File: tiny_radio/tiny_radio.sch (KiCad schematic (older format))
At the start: 9 parts, among them IC1 ATTINY84-P, P1 CONN_4, P2 CONN_3X2, P3 CONN_2, U1 RFM12B

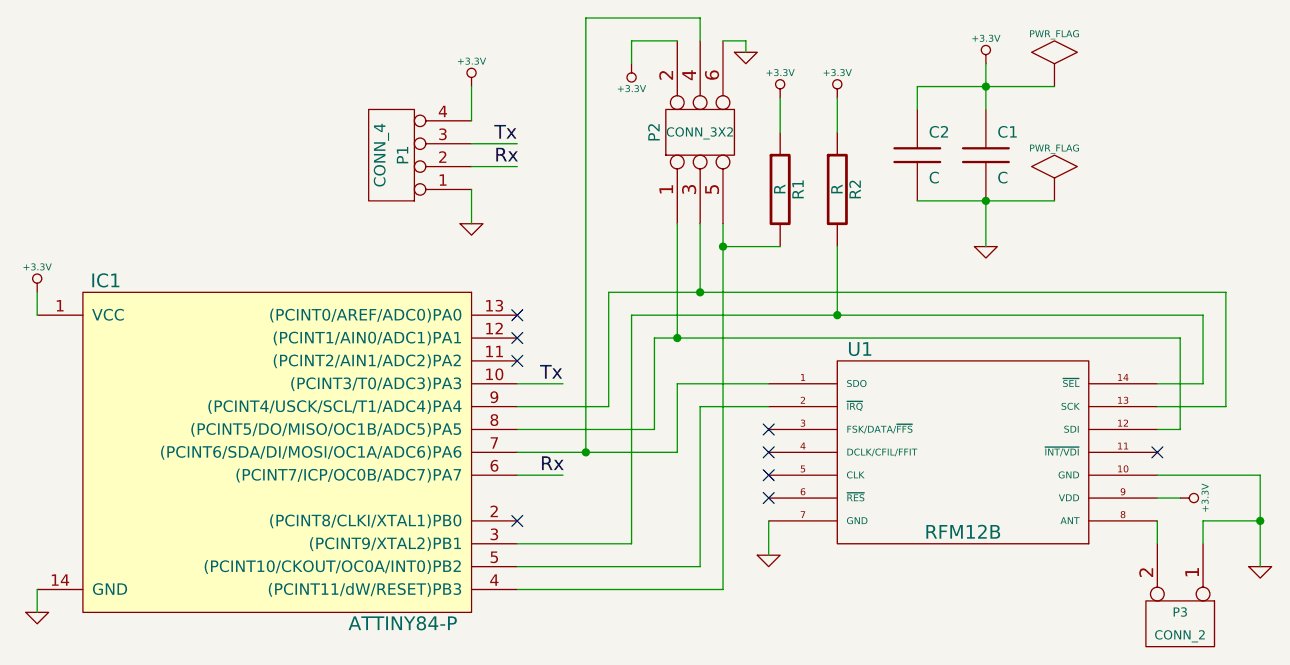
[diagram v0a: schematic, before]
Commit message: moved block over
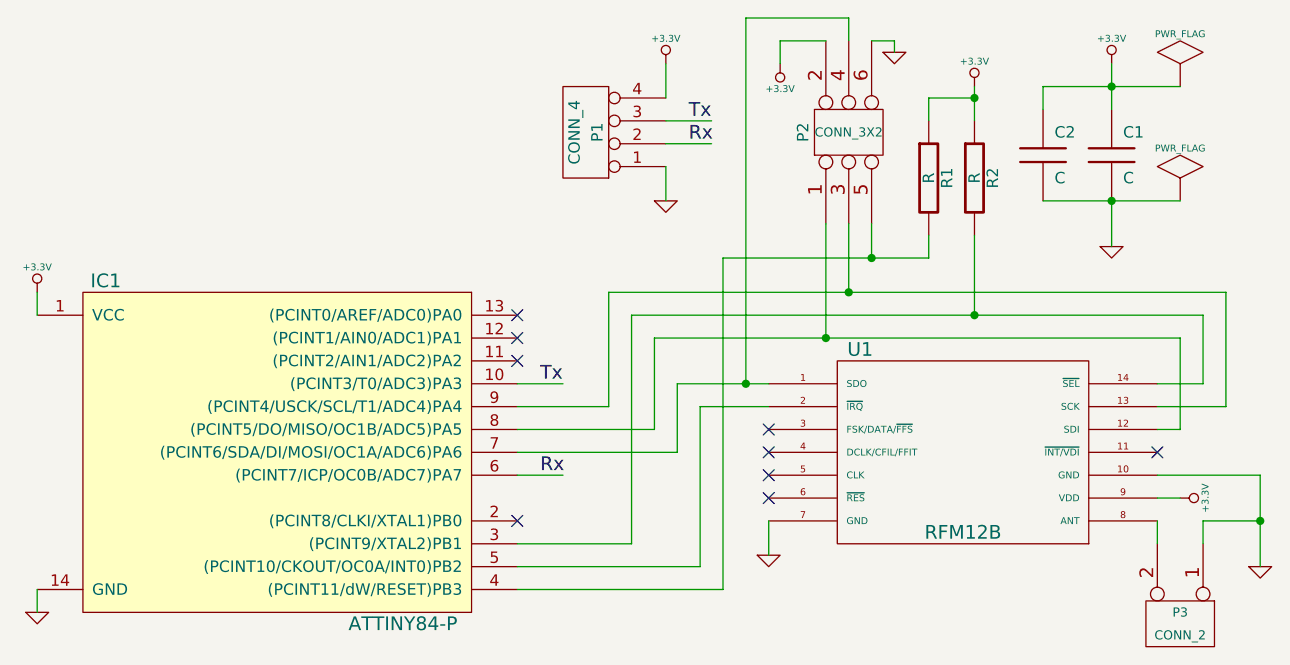
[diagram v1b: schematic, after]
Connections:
- wire segments 56 -> 59
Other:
- moved on the sheet: C1, C2, P1, P2, R1, R2
